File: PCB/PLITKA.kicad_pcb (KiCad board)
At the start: 2 copper layers, 120.5 x 85.5 mm, 56 parts, among them SW1 MX_SW_HS, SW10 MX_SW_HS, SW11 MX_SW_HS, SW12 MX_SW_HS, SW13 MX_SW_HS, SW14 MX_SW_HS, SW15 MX_SW_HS, SW16 MX_SW_HS, SW17 MX_SW_HS, SW18 RotaryEncoder, SW2 MX_SW_HS, SW3 MX_SW_HS, SW4 MX_SW_HS, SW5 MX_SW_HS, SW6 MX_SW_HS, SW7 MX_SW_HS, SW8 MX_SW_HS, SW9 MX_SW_HS, U1 nice!nano

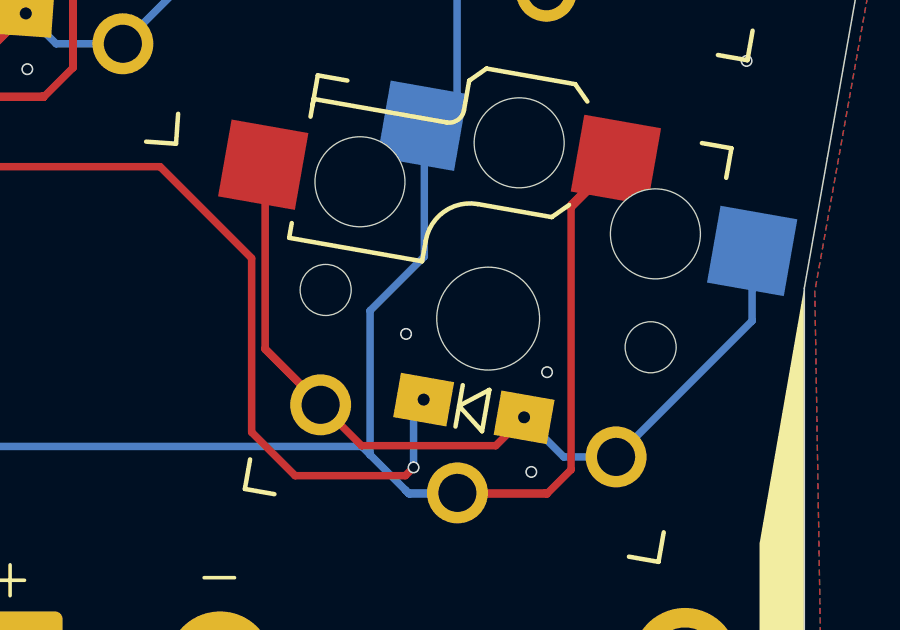
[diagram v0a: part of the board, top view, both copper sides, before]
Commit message: KiCad versions update
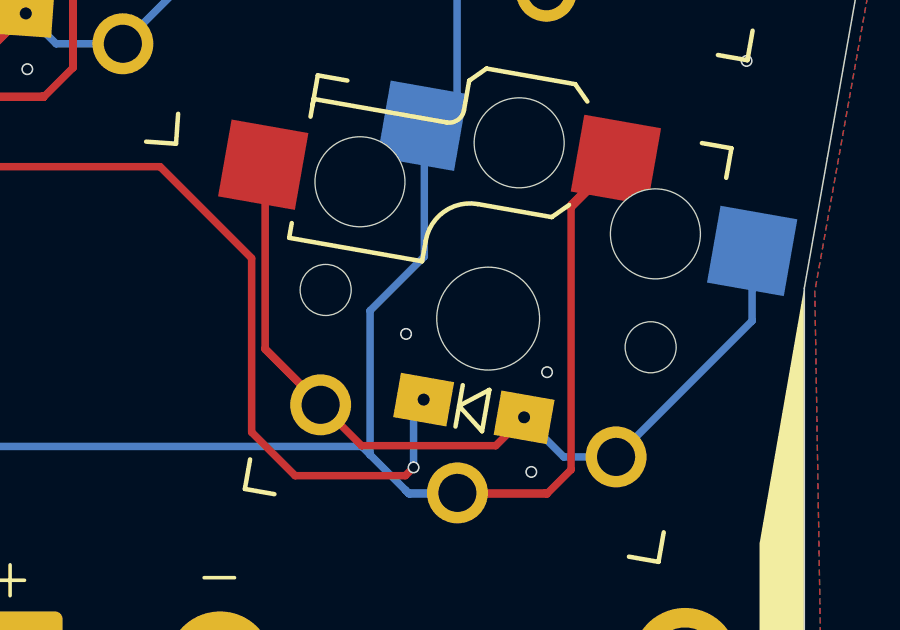
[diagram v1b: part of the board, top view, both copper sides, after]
